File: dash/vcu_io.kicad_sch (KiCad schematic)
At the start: 38 parts, among them J10 Conn_02x01, J11 Conn_02x02_Top_Bottom, J5 M80-5102042, J6 Conn_02x02_Top_Bottom, J7 Conn_02x01, J8 Conn_02x02_Top_Bottom, J9 Conn_02x01, Q2 XP262N7002TR-G, Q3 XP262N7002TR-G, Q4 XP262N7002TR-G, Q5 XP262N7002TR-G, U10 TCAN3404-Q1, U9 TCAN3404-Q1

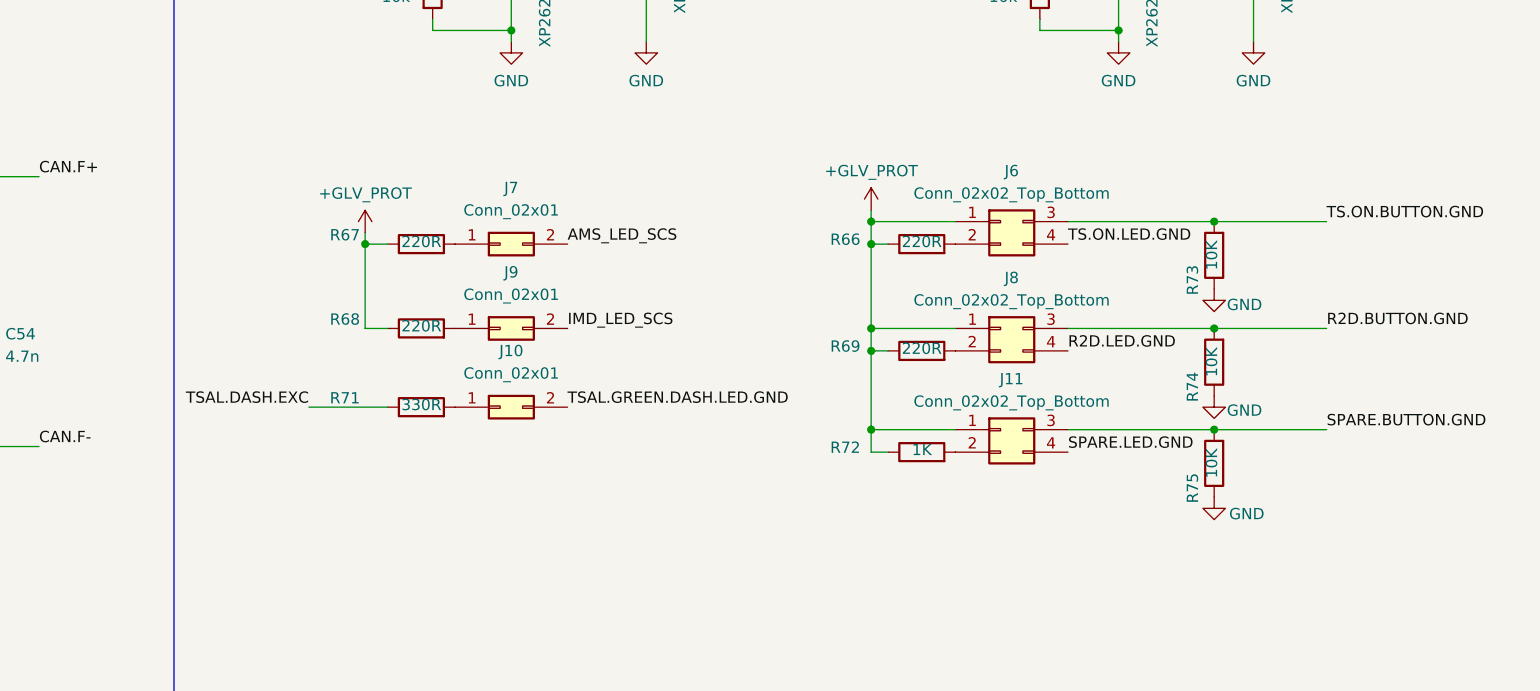
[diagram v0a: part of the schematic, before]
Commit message: Adding silkscreen, cleaning up DRC
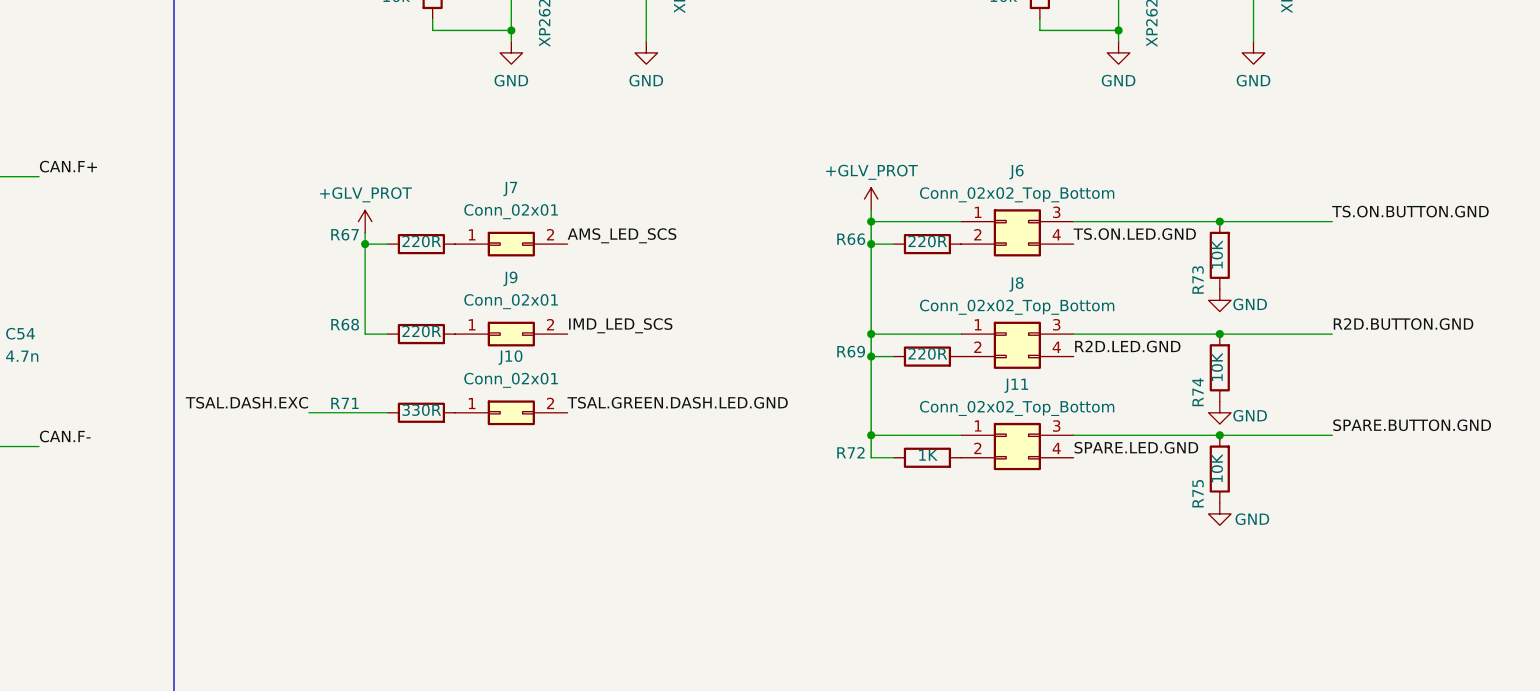
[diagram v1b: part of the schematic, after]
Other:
- moved on the sheet: J10, J11, J6, J8, J9, R66, R68, R69, R71, R72, R73, R74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
